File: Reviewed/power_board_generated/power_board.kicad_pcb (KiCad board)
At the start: 8 copper layers, 34 x 34 mm, 116 parts

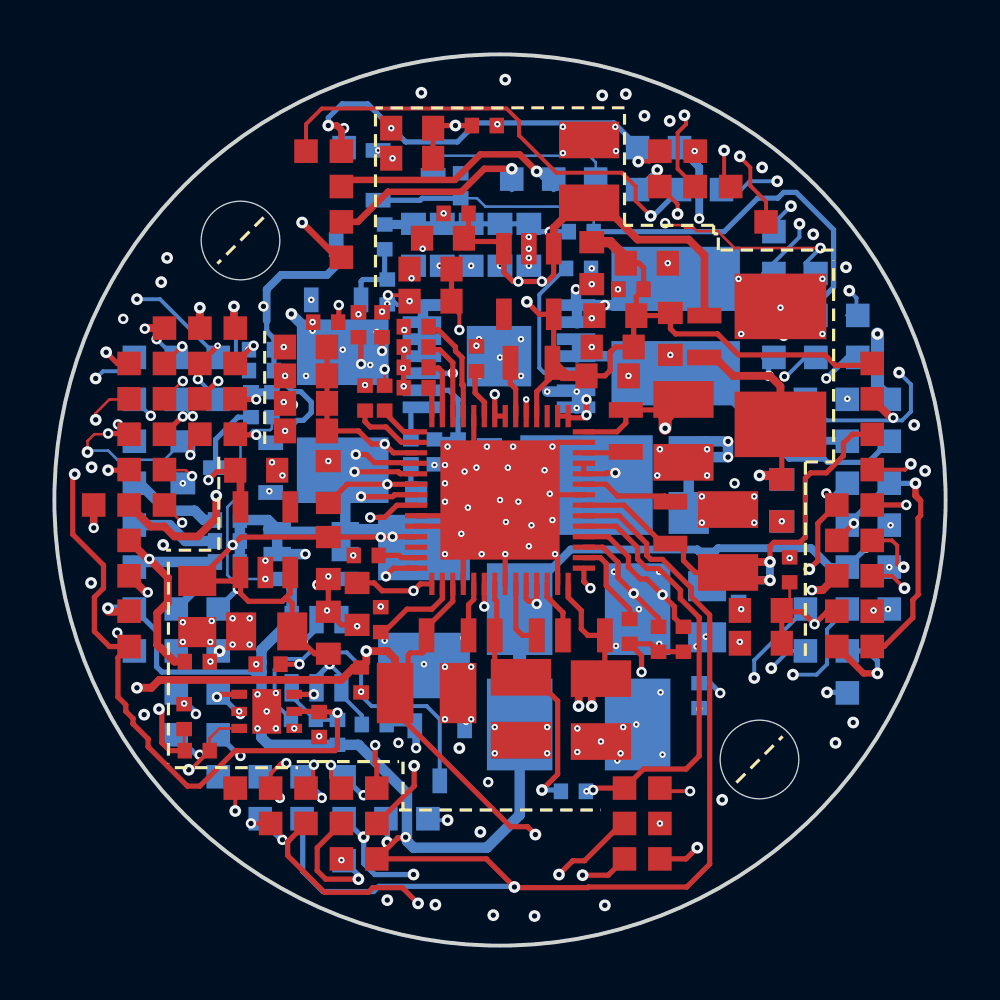
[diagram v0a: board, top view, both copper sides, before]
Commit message: fixed lga pad corrections
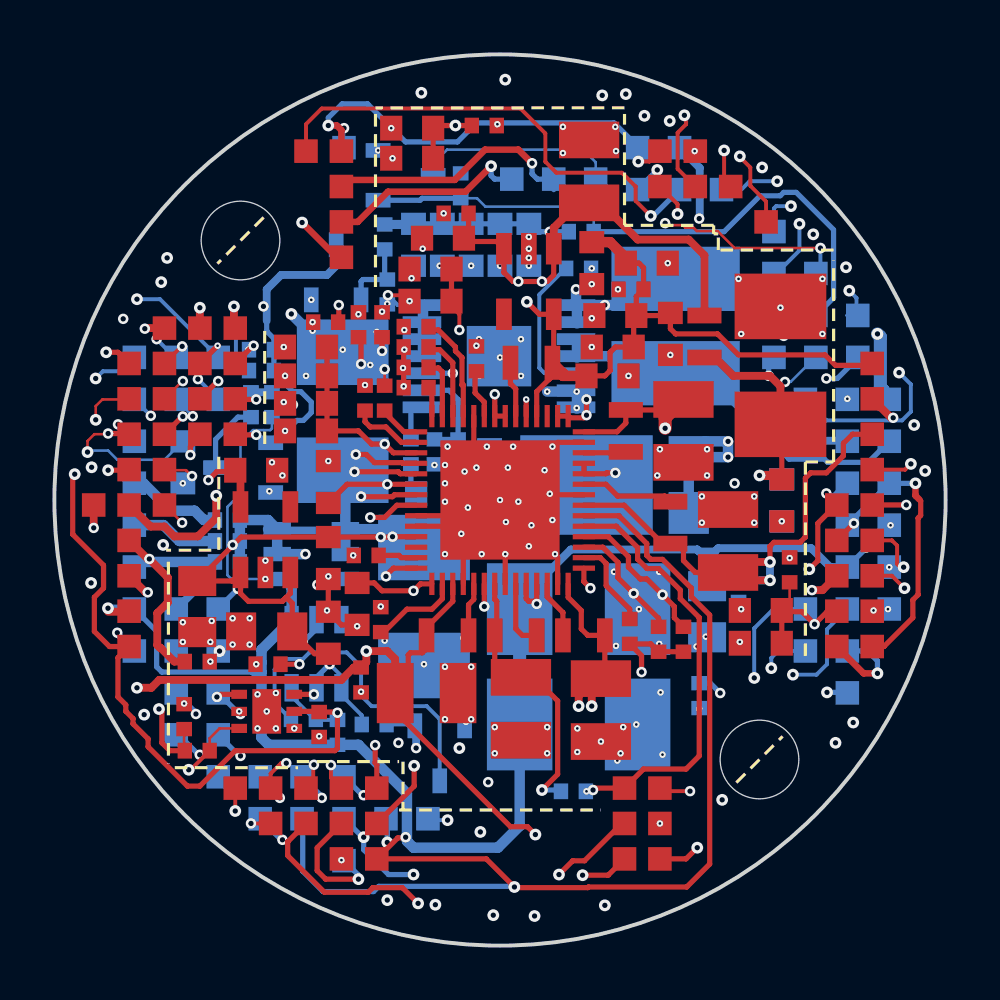
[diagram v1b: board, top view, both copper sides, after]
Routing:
- net WBA_BOOT0: track 45.3 -> 46.1 mm
- net WBA_HCI_MISO: track 51.1 -> 51.9 mm
- net SYS_SPI_MISO: track 37.3 -> 36.7 mm
- net MAG_DRDY: track 9.19 -> 9.79 mm
